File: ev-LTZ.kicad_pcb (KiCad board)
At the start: 2 copper layers, 50 x 100 mm, 36 parts, among them P1 VIN+, P2 CONN_01X02, P3 VH-, P4 VH+, P5 SENSE-, P6 SENSE+, P7 VIN-, Q1 BD139, U1 LT1013N8

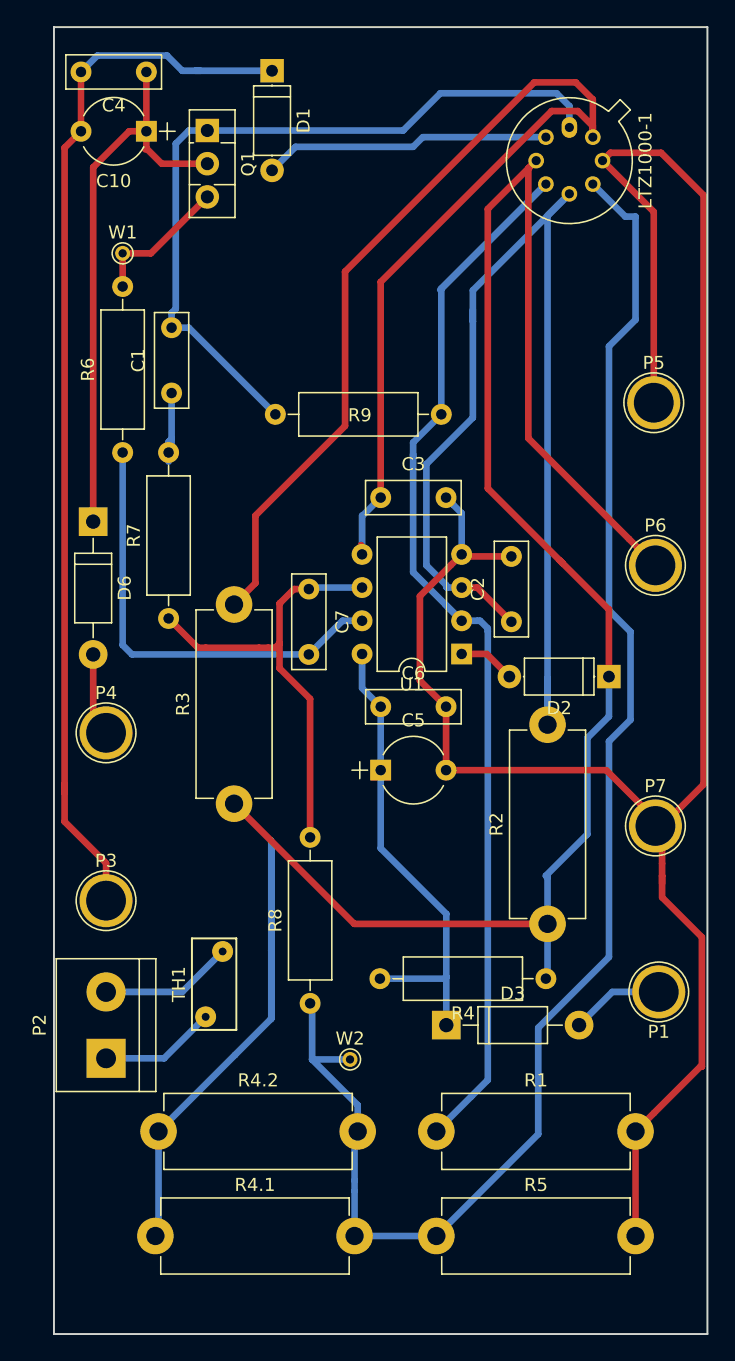
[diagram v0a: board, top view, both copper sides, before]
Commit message: finish pcb
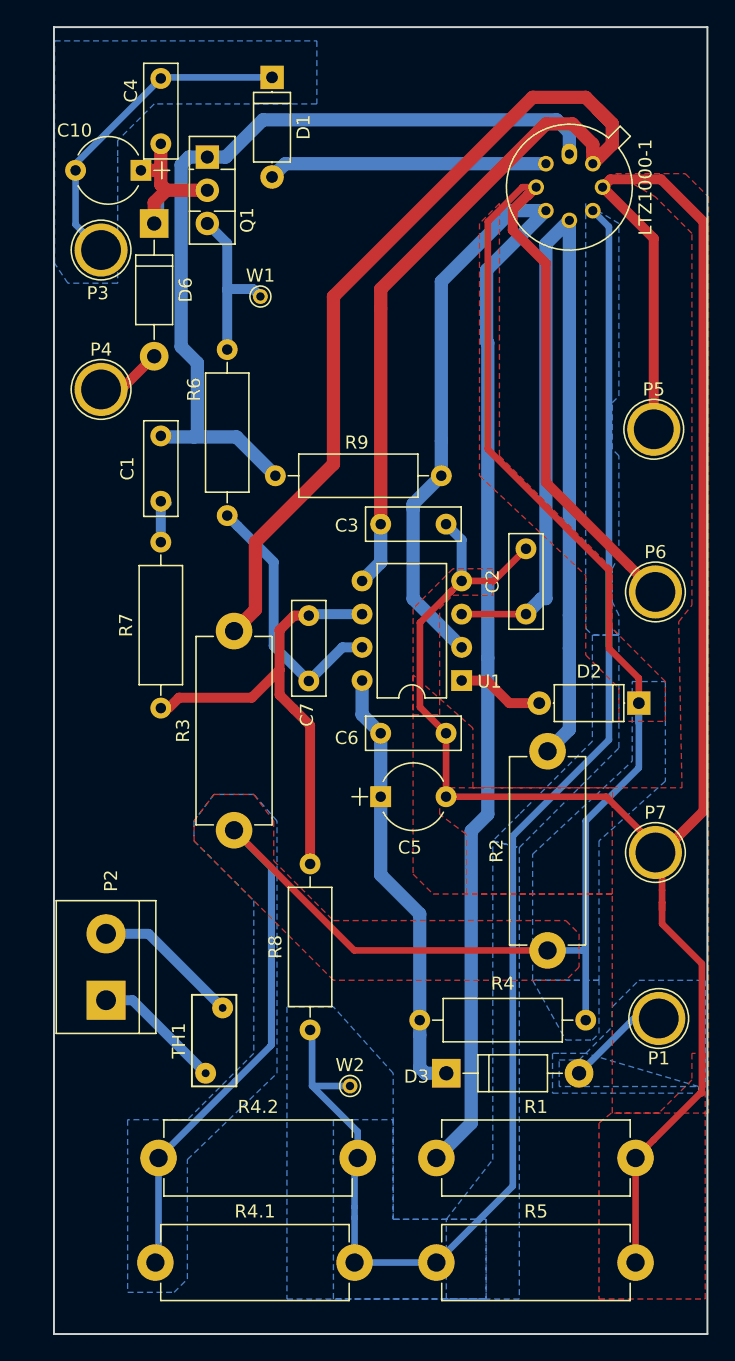
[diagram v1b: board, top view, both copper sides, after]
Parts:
- moved P3 49.8 mm to (133.6, 67.1)
- moved P4 26.3 mm to (133.6, 77.7)
- moved D6 23.3 mm to (137.7, 65.0)
- moved W1 11.0 mm to (145.8, 70.6)
- moved R6 9.34 mm to (143.3, 87.4)
- moved C1 8.32 mm to (138.2, 86.3)
- moved R7 6.88 mm to (138.2, 102.1)
- moved C4 5.61 mm to (138.2, 58.9), turned to 90 degrees
- moved R9 4.70 mm to (159.6, 84.3)
- moved P2 4.45 mm to (134.0, 124.5)
- moved R4 4.40 mm to (170.7, 126.0)
- moved TH1 4.32 mm to (142.9, 125.0)
- moved D3 3.68 mm to (160.0, 130.0)
- moved D2 3.06 mm to (174.8, 101.7)
- moved C10 3.02 mm to (136.7, 61.0)
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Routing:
- net /VH-: track 81.9 -> 25.2 mm
- net Net-(C10-Pad1): track 43.4 -> 19.1 mm
- net Net-(LTZ1000-1-Pad4): track 95.0 -> 118.7 mm
- net Net-(C7-Pad2): track 34.5 -> 20.4 mm
- net Net-(C3-Pad1): track 101.3 -> 110.7 mm
- net Net-(C2-Pad1): track 87.1 -> 79.1 mm
- net /SENSE+: track 184.9 -> 192.5 mm
- net Net-(C1-Pad2): track 59.0 -> 64.5 mm
- net /TSENSE: track 118.6 -> 115.1 mm
- net Net-(C1-Pad1): track 6.49 -> 3.08 mm
- net Net-(C5-Pad1): track 36.9 -> 33.7 mm
- net GND: track 160.1 -> 162.4 mm
- net Net-(D2-Pad2): track 4.37 -> 6.65 mm
- net /HEAT: track 11.0 -> 13.1 mm
- net /VH+: track 6.62 -> 5.12 mm
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- added copper zone on B.Cu, net /SENSE+
- added copper zone on F.Cu, net /SENSE+
- added copper zone on B.Cu, net /TSENSE
- added copper zone on B.Cu, net /VH-
- added copper zone on B.Cu, net /VIN+
- added copper zone on F.Cu, net GND
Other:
- net class Default: trace_width 0.508 -> 0.762
- net class Power added: clearance 0.2, trace_width 1.016, via_dia 0.6, via_drill 0.4
